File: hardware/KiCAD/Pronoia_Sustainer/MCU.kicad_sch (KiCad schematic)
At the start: 8 parts, among them Q6 AO3400A, U2 Teensy4.1

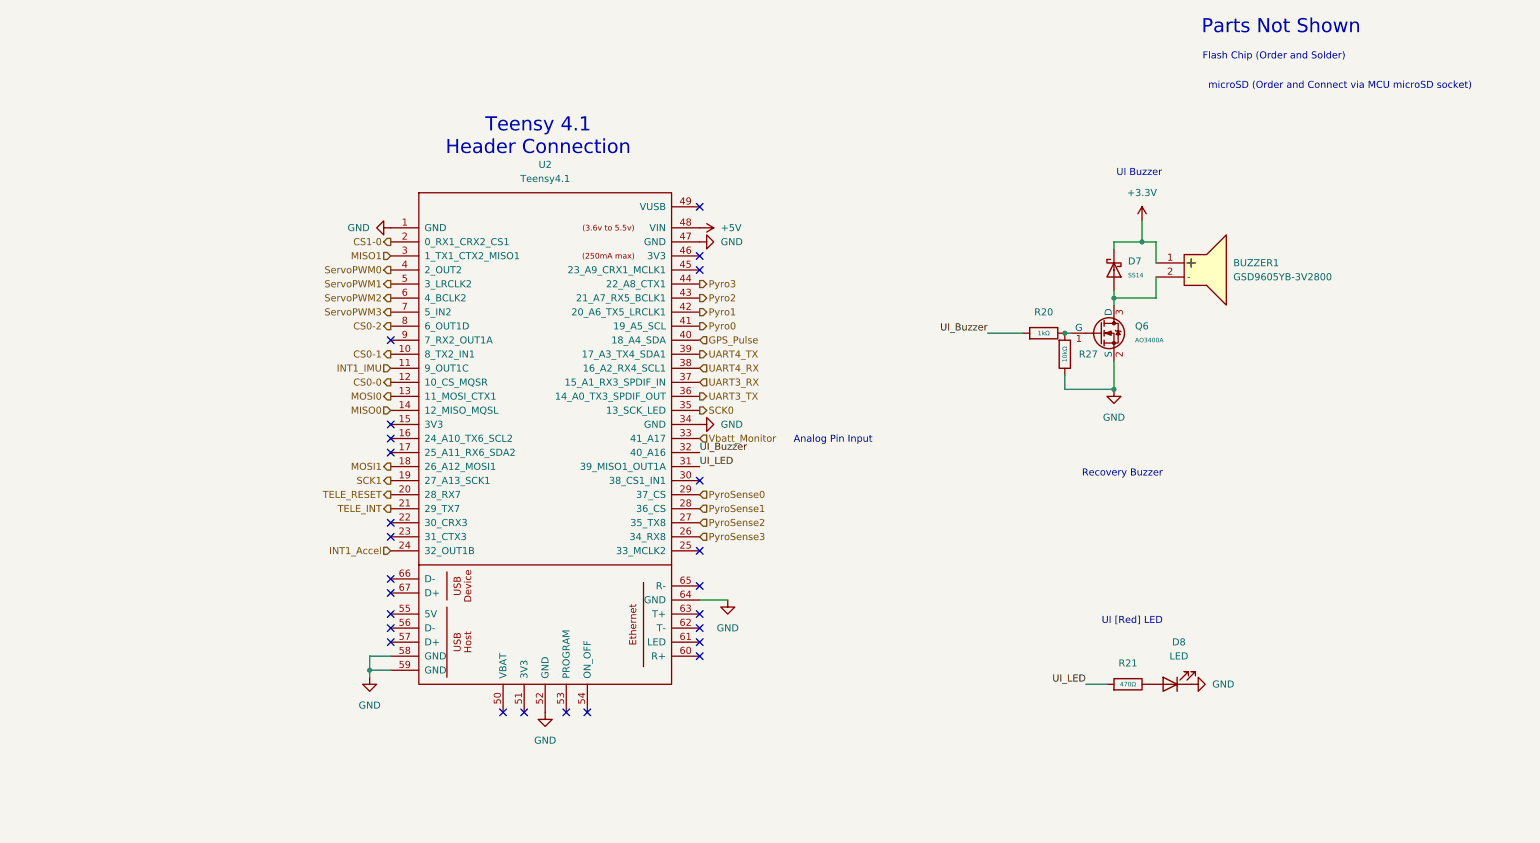
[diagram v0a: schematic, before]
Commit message: Finalized v2.0 of Pronoia Schematic
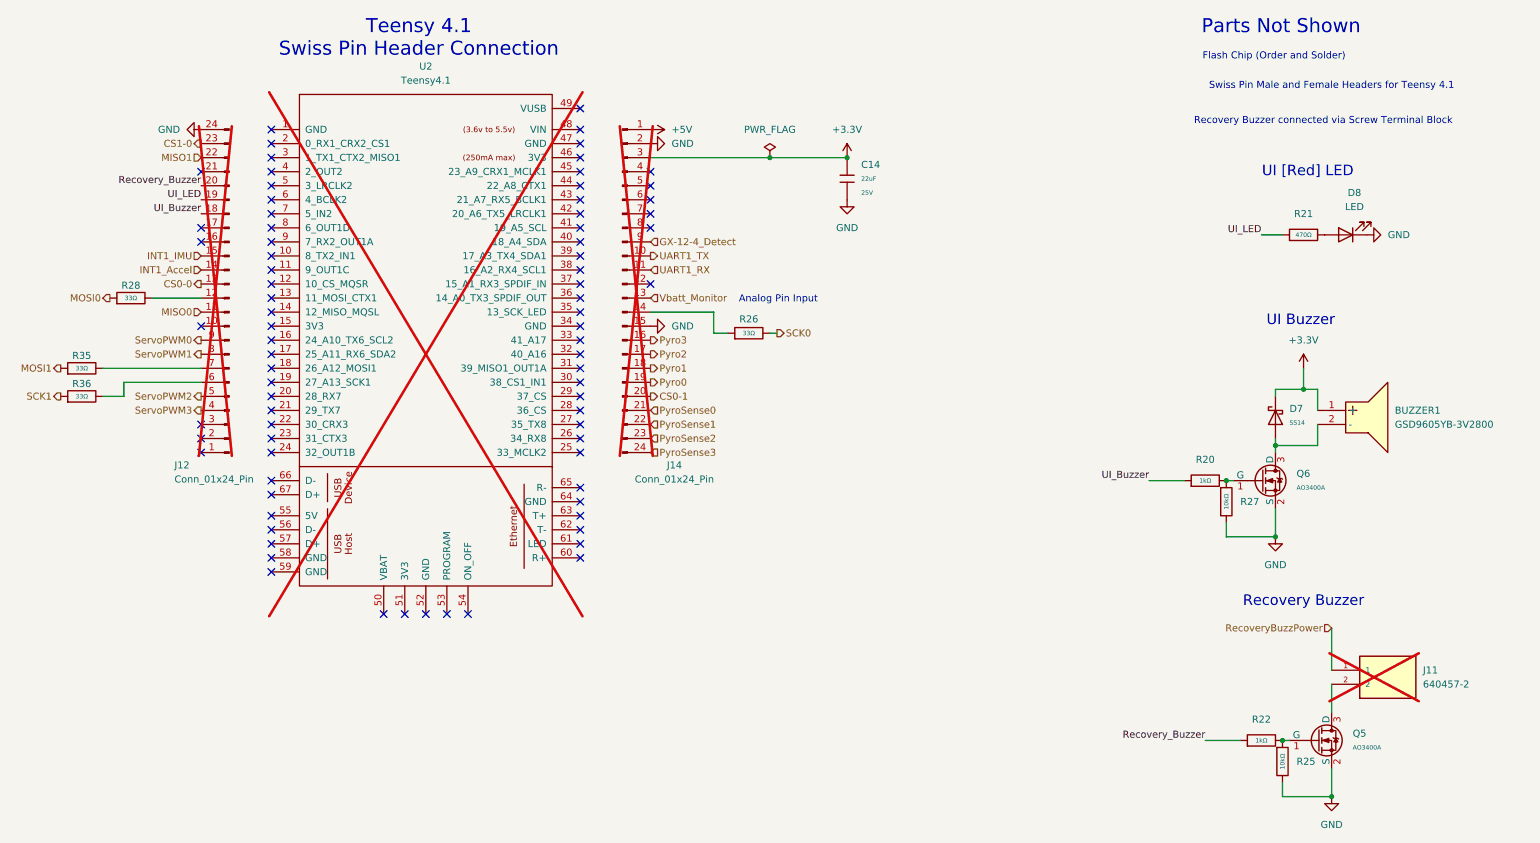
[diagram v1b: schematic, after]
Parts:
- added C14: 22uF, PCM_JLCPCB:C_0805, symbol PCM_JLCPCB-Capacitors:0805,22uF
- added J11: 640457-2, 640457-2:TE_640457-2, symbol 640457-2:640457-2
- added J12, J14: Conn_01x24_Pin, Connector_PinSocket_2.54mm:PinSocket_1x24_P2.54mm_Vertical, symbol Connector:Conn_01x24_Pin
- added Q5: AO3400A, PCM_JLCPCB:Q_SOT-23, symbol PCM_JLCPCB-Transistors:NMOS,AO3400A
- added R22: 1kΩ, PCM_JLCPCB:R_0805, symbol PCM_JLCPCB-Resistors:0805,1kΩ
- added R25: 10kΩ, PCM_JLCPCB:R_0805, symbol PCM_JLCPCB-Resistors:0805,10kΩ
- added R26, R28, R35, R36: 33Ω, PCM_JLCPCB:R_0402, symbol PCM_JLCPCB-Resistors:0402,33Ω
- D8: footprint (none) -> LED_SMD:LED_0603_1608Metric; LCSC (none) -> C3030991
- U2: now not fitted
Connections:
- net +3.3V: now also C14.1, J14.3 (Pin_3)
- net +5V: now also J14.1 (Pin_1); no longer U2.48 (VIN)
- net CS0-0: now also J12.13 (Pin_13); no longer U2.12 (10_CS_MQSR)
- net CS0-1: now also J14.20 (Pin_20); no longer U2.10 (8_TX2_IN1)
- net CS1-0: now also J12.23 (Pin_23); no longer U2.2 (0_RX1_CRX2_CS1)
- net GND: now also C14.2, J12.24 (Pin_24), J14.15 (Pin_15), J14.2 (Pin_2), Q5.2 (S), R25.2; no longer U2.1 (GND), U2.34 (GND), U2.47 (GND), U2.52 (GND), U2.58 (GND), U2.59 (GND), U2.64 (GND)
- net INT1_Accel: now also J12.14 (Pin_14); no longer U2.24 (32_OUT1B)
- net INT1_IMU: now also J12.15 (Pin_15); no longer U2.11 (9_OUT1C)
- net MISO0: now also J12.11 (Pin_11); no longer U2.14 (12_MISO_MQSL)
- net MISO1: now also J12.22 (Pin_22); no longer U2.3 (1_TX1_CTX2_MISO1)
- net MOSI0: now also R28.1; no longer U2.13 (11_MOSI_CTX1)
- net MOSI1: now also R35.1; no longer U2.18 (26_A12_MOSI1)
- net Pyro0: now also J14.19 (Pin_19); no longer U2.41 (19_A5_SCL)
- net Pyro1: now also J14.18 (Pin_18); no longer U2.42 (20_A6_TX5_LRCLK1)
- net Pyro2: now also J14.17 (Pin_17); no longer U2.43 (21_A7_RX5_BCLK1)
- net Pyro3: now also J14.16 (Pin_16); no longer U2.44 (22_A8_CTX1)
- net PyroSense0: now also J14.21 (Pin_21); no longer U2.29 (37_CS)
- net PyroSense1: now also J14.22 (Pin_22); no longer U2.28 (36_CS)
- net PyroSense2: now also J14.23 (Pin_23); no longer U2.27 (35_TX8)
- net PyroSense3: now also J14.24 (Pin_24); no longer U2.26 (34_RX8)
- net SCK0: now also R26.2; no longer U2.35 (13_SCK_LED)
- net SCK1: now also R36.1; no longer U2.19 (27_A13_SCK1)
- net ServoPWM0: now also J12.9 (Pin_9); no longer U2.4 (2_OUT2)
- net ServoPWM1: now also J12.8 (Pin_8); no longer U2.5 (3_LRCLK2)
- net ServoPWM2: now also J12.5 (Pin_5); no longer U2.6 (4_BCLK2)
- net ServoPWM3: now also J12.4 (Pin_4); no longer U2.7 (5_IN2)
- net UI_Buzzer: now also J12.18 (Pin_18); no longer U2.32 (40_A16)
- net UI_LED: now also J12.19 (Pin_19); no longer U2.31 (39_MISO1_OUT1A)
- net Vbatt_Monitor: now also J14.13 (Pin_13); no longer U2.33 (41_A17)
- net CS0-2: no longer names the net of U2.8 (6_OUT1D)
- net GPS_Pulse: no longer names the net of U2.40 (18_A4_SDA)
- net TELE_INT: no longer names the net of U2.21 (29_TX7)
- net TELE_RESET: no longer names the net of U2.20 (28_RX7)
- net UART3_RX: no longer names the net of U2.37 (15_A1_RX3_SPDIF_IN)
- net UART3_TX: no longer names the net of U2.36 (14_A0_TX3_SPDIF_OUT)
- net UART4_RX: no longer names the net of U2.38 (16_A2_RX4_SCL1)
- net UART4_TX: no longer names the net of U2.39 (17_A3_TX4_SDA1)
- new net: Q5.1 (G), R22.2, R25.1
- new net: J11.2, Q5.3 (D)
- new net: J12.7 (Pin_7), R35.2
- new net: J14.14 (Pin_14), R26.1
- new net: J12.12 (Pin_12), R28.2
- new net: J12.6 (Pin_6), R36.2
- new net GX-12-4_Detect: J14.9 (Pin_9)
- new net RecoveryBuzzPower: J11.1
- new net Recovery_Buzzer: J12.20 (Pin_20), R22.1
- new net UART1_RX: J14.11 (Pin_11)
- new net UART1_TX: J14.10 (Pin_10)
- no-connect marks 25 -> 80
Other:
- note added: "Recovery Buzzer connected via Screw Terminal Block"
- note added: "Swiss Pin Male and Female Headers for Teensy 4.1"
- note added: "Teensy 4.1 Swiss Pin Header Connection"
- note removed: "Teensy 4.1 Header Connection"
- note removed: "microSD (Order and Connect via MCU microSD socket)"
- moved on the sheet: D7, D8, Q6, R20, R21, R27
